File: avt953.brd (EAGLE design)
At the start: 100 x 80 mm, 51 parts, among them CON3 RJ45-6L2-B, CON4A MKDS_5/3-6,35, CON4B MKDS_5/3-6,35, CON4C MKDS_5/3-6,35, CON4D MKDS_5/3-6,35, X1 20MHz, X2 20MHz

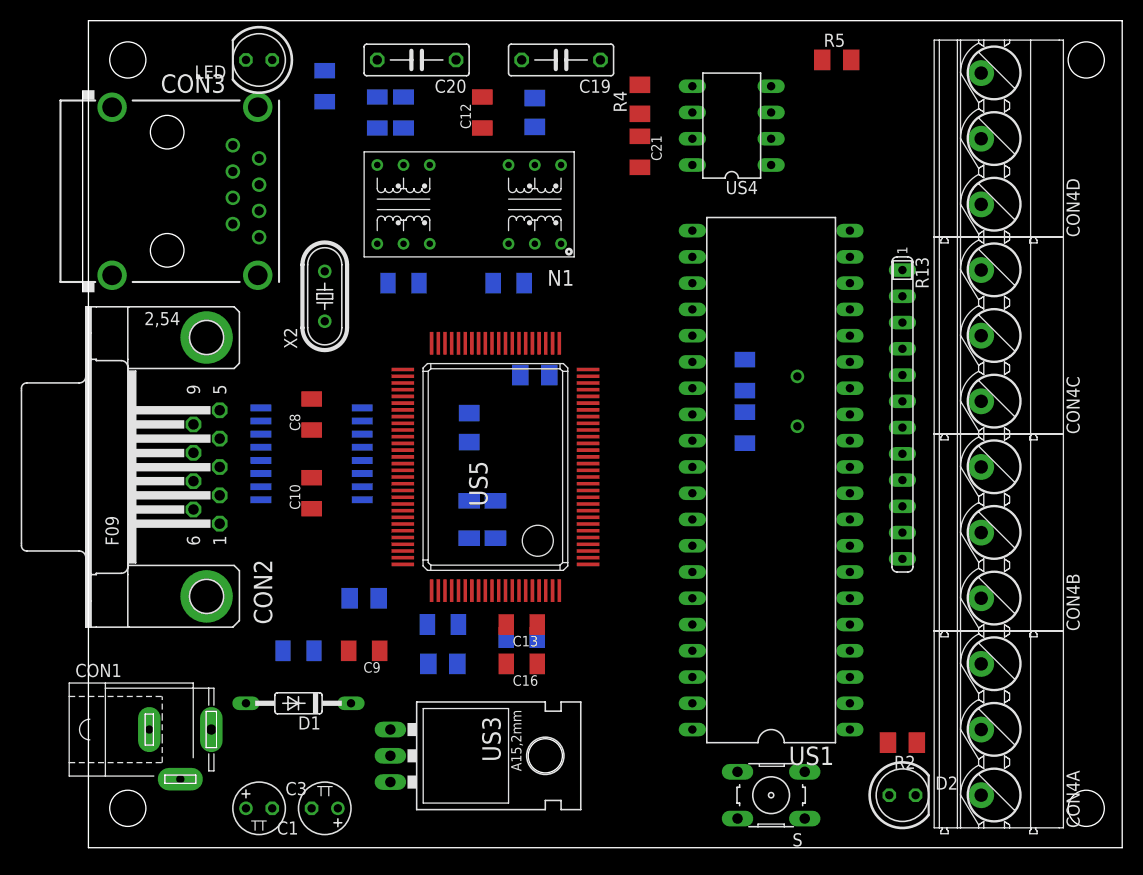
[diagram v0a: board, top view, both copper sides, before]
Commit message: Przepuszczono płytkę jeszcze raz przez autorouter, rozluźniając kryteria dodania przelotek i zmiany kierunku ścieżek. Brzydko wyszło, ale wynik 100%.
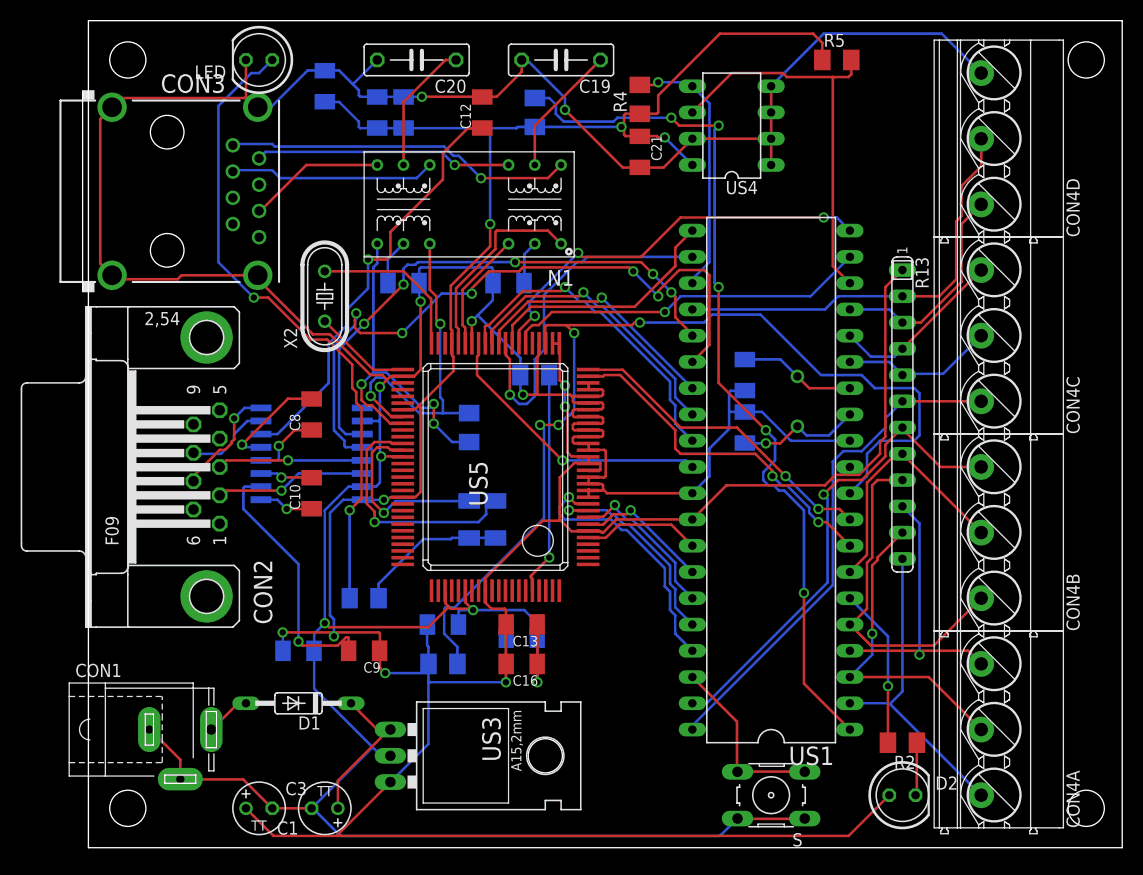
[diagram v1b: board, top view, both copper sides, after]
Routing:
- net GND: track 0.00 -> 452.1 mm, vias 0 -> 10
- net VCC: track 0.00 -> 349.7 mm, vias 0 -> 10
- net RESET: track 0.00 -> 96.6 mm, vias 0 -> 4
- net N$35: track 0.00 -> 85.3 mm, vias 0 -> 5
- net RXD: track 0.00 -> 66.6 mm, vias 0 -> 5
- net N$31: track 0.00 -> 62.7 mm, vias 0 -> 2
- net TXD: track 0.00 -> 52.9 mm, vias 0 -> 5
- net IN6: track 0.00 -> 48.8 mm
- net IN5: track 0.00 -> 46.8 mm, vias 0 -> 1
- net IN10: track 0.00 -> 41.3 mm
- net N$2: track 0.00 -> 41.3 mm, vias 0 -> 1
- net SD1: track 0.00 -> 40.2 mm, vias 0 -> 3
- net N$37: track 0.00 -> 39.2 mm
- net SD0: track 0.00 -> 35.5 mm, vias 0 -> 1
- net SD3: track 0.00 -> 34.3 mm, vias 0 -> 1
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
